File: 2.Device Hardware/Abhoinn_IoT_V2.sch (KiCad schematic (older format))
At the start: 46 parts, among them IC1 AX-SIP-SFEU-1-01-TX30, IC2 MS5840-02BA01, J1 Conn_01x02, J2 Conn_01x02, J3 Conn_02x05_Odd_Even, J4 Conn_02x05_Odd_Even, J5 Conn_Coaxial, J6 Conn_01x02_Female, P1 USB_C_Plug_USB2.0, U1 XC6206PxxxMR, U2 USBLC6-2SC6, U3 STM32L082KZTx

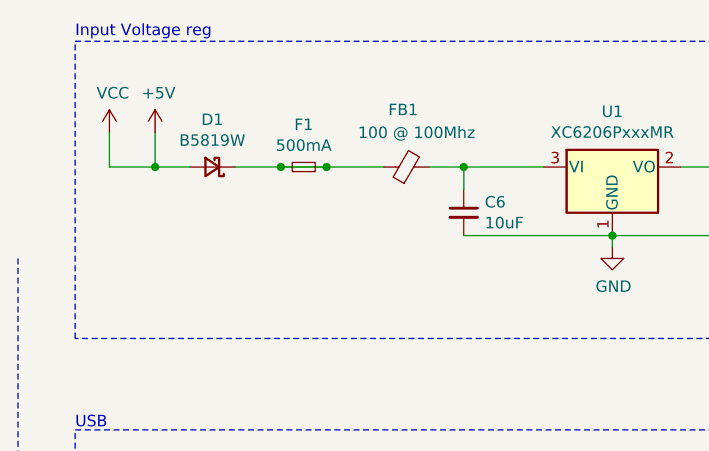
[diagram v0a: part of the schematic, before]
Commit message: update
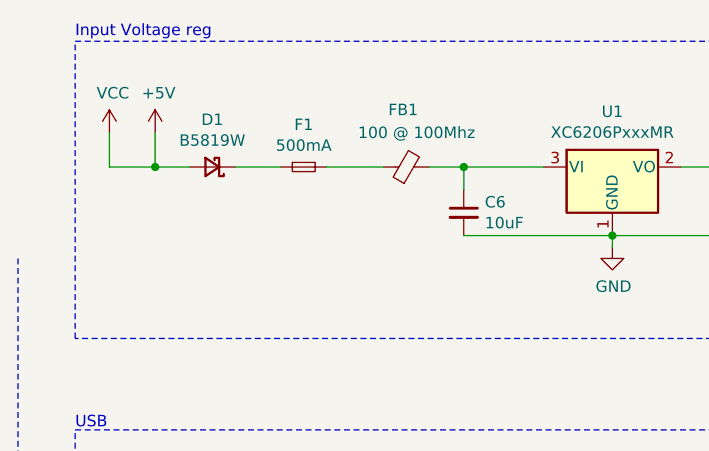
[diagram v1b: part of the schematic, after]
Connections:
- wire segments 111 -> 110
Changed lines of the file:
@@
 	2000 2900 2000 2850
 NoConn ~ 1850 2900
-Wire Wire Line
-	1550 1350 1750 1350
-Connection ~ 1750 1350
 $Comp
 L power:+5V #PWR0136
@@
 Wire Wire Line
 	1350 1350 1550 1350
-Connection ~ 1550 1350
 Text GLabel 6000 3200 2    50   Input ~ 0
 LPUART1_TX
